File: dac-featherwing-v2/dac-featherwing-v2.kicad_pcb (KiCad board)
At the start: 2 copper layers, 44.5 x 58.4 mm, 36 parts, among them J1 BOT, J2 TOP, J3 AudioJack4, J4 AudioJack4, U1 WM8731CLSEFL

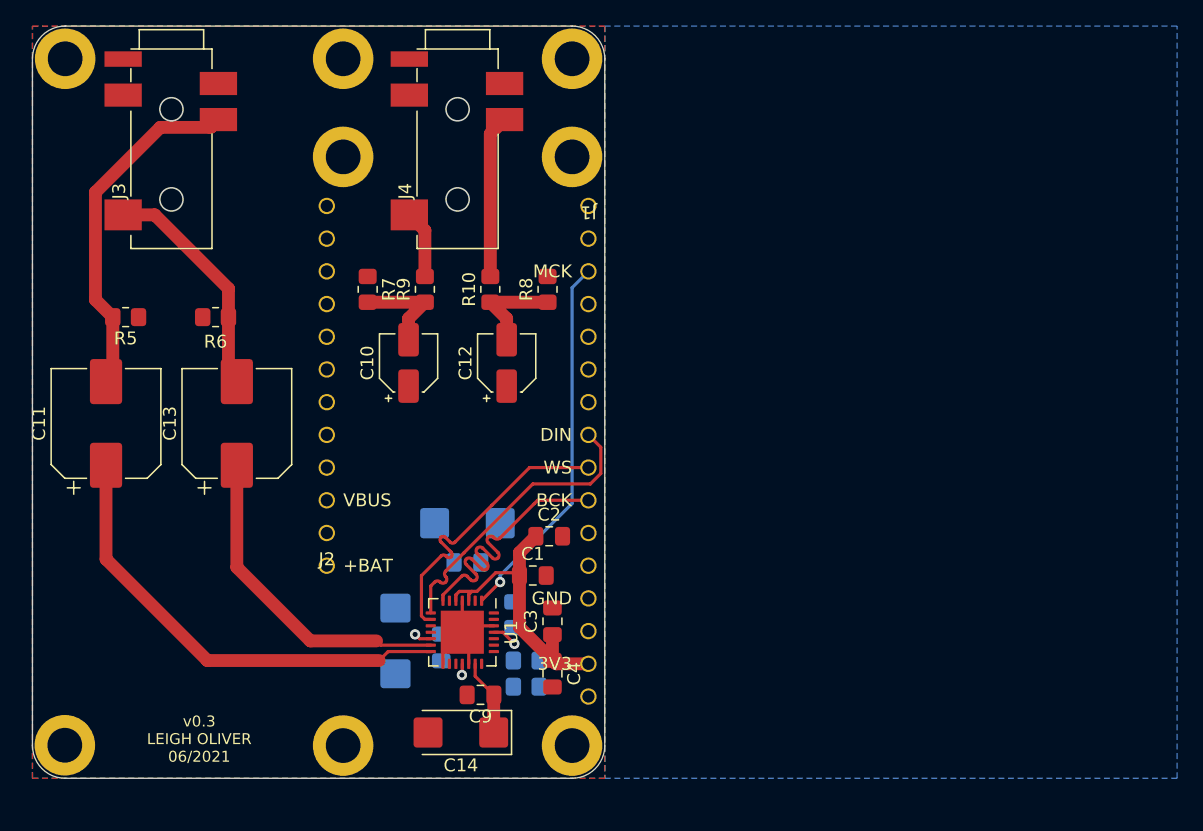
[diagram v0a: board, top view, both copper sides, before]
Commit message: Full route #1 complete
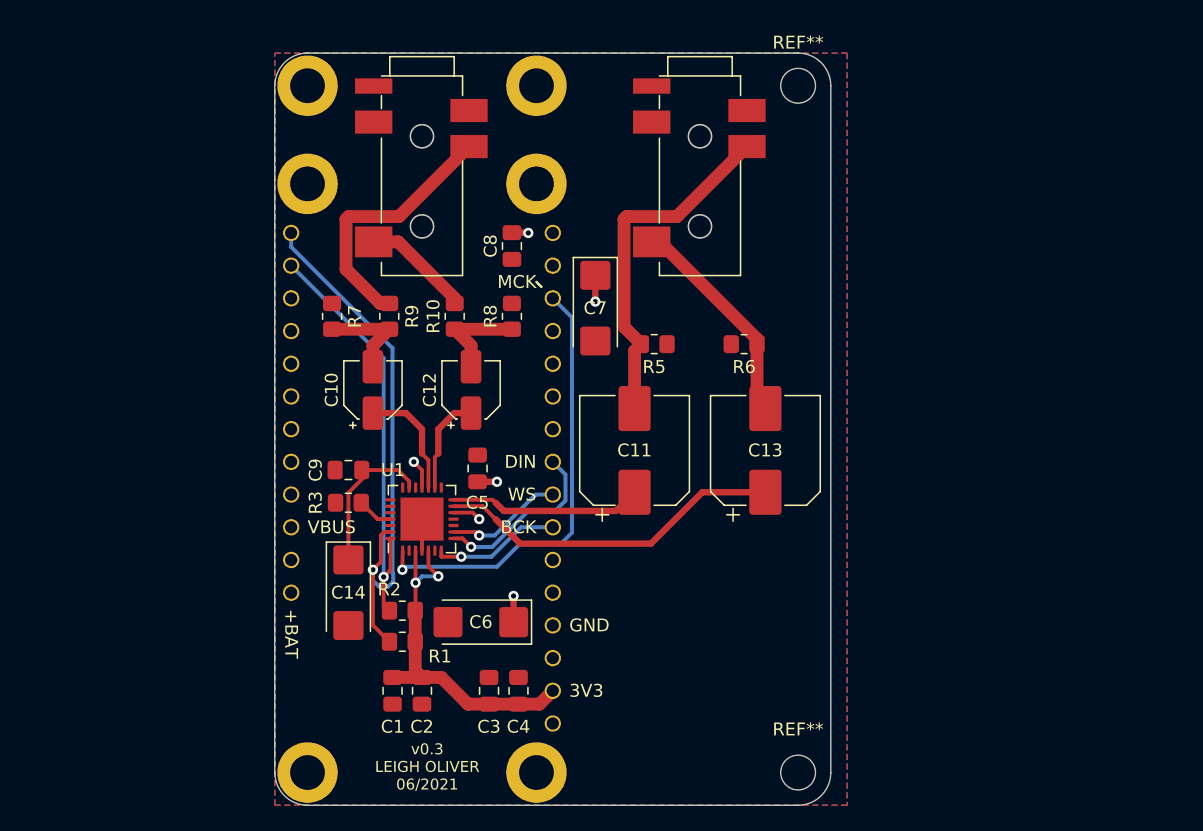
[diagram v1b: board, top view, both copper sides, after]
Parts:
- removed the REF** at (92.7, 55.9)
- removed the REF** at (92.7, 109.2)
- added REF**: MountingHole_2.7mm_M2.5_DIN965, MountingHole:MountingHole_2.7mm_M2.5_DIN965, F.Cu at (149.6, 58.0)
- added REF**: MountingHole_2.7mm_M2.5_DIN965, MountingHole:MountingHole_2.7mm_M2.5_DIN965, F.Cu at (149.6, 111.3)
- C5, C6, C7, C8, R1, R2, R3: moved to F.Cu
- moved J3 41.1 mm to (142.0, 68.9)
- moved R6 41.1 mm to (145.4, 78.0)
- moved C11 41.1 mm to (136.9, 86.3)
- moved C13 41.1 mm to (147.1, 86.3)
- moved R5 41.1 mm to (138.5, 78.0)
- moved C8 24.8 mm to (127.4, 70.4), turned to -90 degrees
- moved C9 20.3 mm to (114.7, 87.8)
- moved C7 19.4 mm to (133.9, 75.2), turned to -90 degrees
- moved C2 15.5 mm to (120.4, 105.0), turned to -90 degrees
- moved R3 15.5 mm to (114.7, 90.4), turned to 180 degrees
- moved C5 14.2 mm to (124.7, 87.7)
- moved C1 14.1 mm to (118.1, 105.0), turned to -90 degrees
- moved C14 13.9 mm to (114.7, 97.3), turned to -90 degrees
- moved R2 11.3 mm to (118.9, 98.7)
- moved R1 9.73 mm to (118.9, 101.2)
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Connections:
- C10 pad 1: Net-(C10-Pad1) -> Net-(U1-Pad17)
- C12 pad 1: Net-(C12-Pad1) -> Net-(U1-Pad16)
- R10 pad 2: ROUT -> LOUT
- R9 pad 2: LOUT -> ROUT
- U1 pad 16: Net-(C10-Pad1) -> Net-(U1-Pad16)
- U1 pad 17: Net-(C12-Pad1) -> Net-(U1-Pad17)
- U1 pad 6: Net-(R4-Pad2) -> unconnected-(U1-Pad6)
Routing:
- net SDA: track 0.00 -> 43.0 mm, vias 0 -> 1
- net SCL: track 0.00 -> 33.3 mm, vias 0 -> 1
- net Net-(C11-Pad1): track 36.1 -> 15.0 mm
- net /I2S_WS: track 22.9 -> 9.14 mm, vias 0 -> 1
- net /I2S_BCK: track 22.8 -> 10.1 mm, vias 0 -> 1
- net +3.3VA: track 2.24 -> 11.3 mm, vias 2 -> 6
- net /I2S_DO: track 23.0 -> 13.9 mm, vias 0 -> 1
- net Net-(U1-Pad17): track 0.00 -> 9.07 mm
- net GND: track 10.8 -> 2.45 mm
- net Net-(U1-Pad16): track 0.00 -> 7.70 mm
- net ROUT: track 12.6 -> 20.2 mm
- net Net-(C14-Pad1): track 5.94 -> 11.9 mm
- net /I2S_MCLK: track 29.0 -> 34.7 mm
- net +3V3: track 23.1 -> 28.1 mm, vias 0 -> 2
- net LOUT: track 5.29 -> 8.50 mm
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- removed copper zone on B.Cu, net GND
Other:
- board size 44.5 x 58.4 mm -> 43.2 x 58.4 mm
